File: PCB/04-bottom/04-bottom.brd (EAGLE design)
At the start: 128 x 129.5 mm, 30 parts, among them CN1 ML8-R, J1 5267-3, J2 5267-3, J3 5267-3, J4 5267-3, J5 22057045, J6 22057045, J7 5267-3

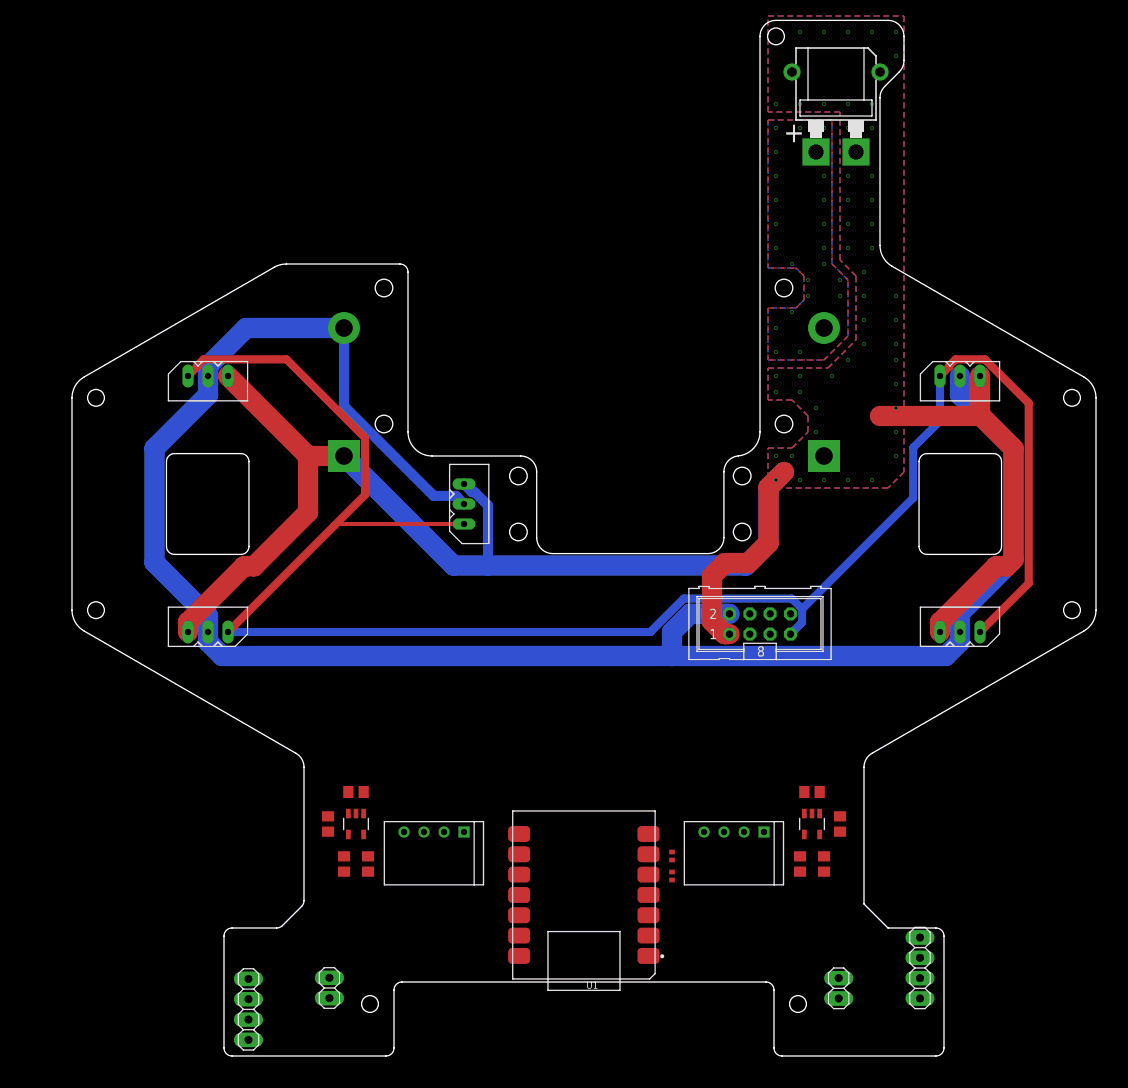
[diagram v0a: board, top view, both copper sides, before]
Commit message: 配線完了！！
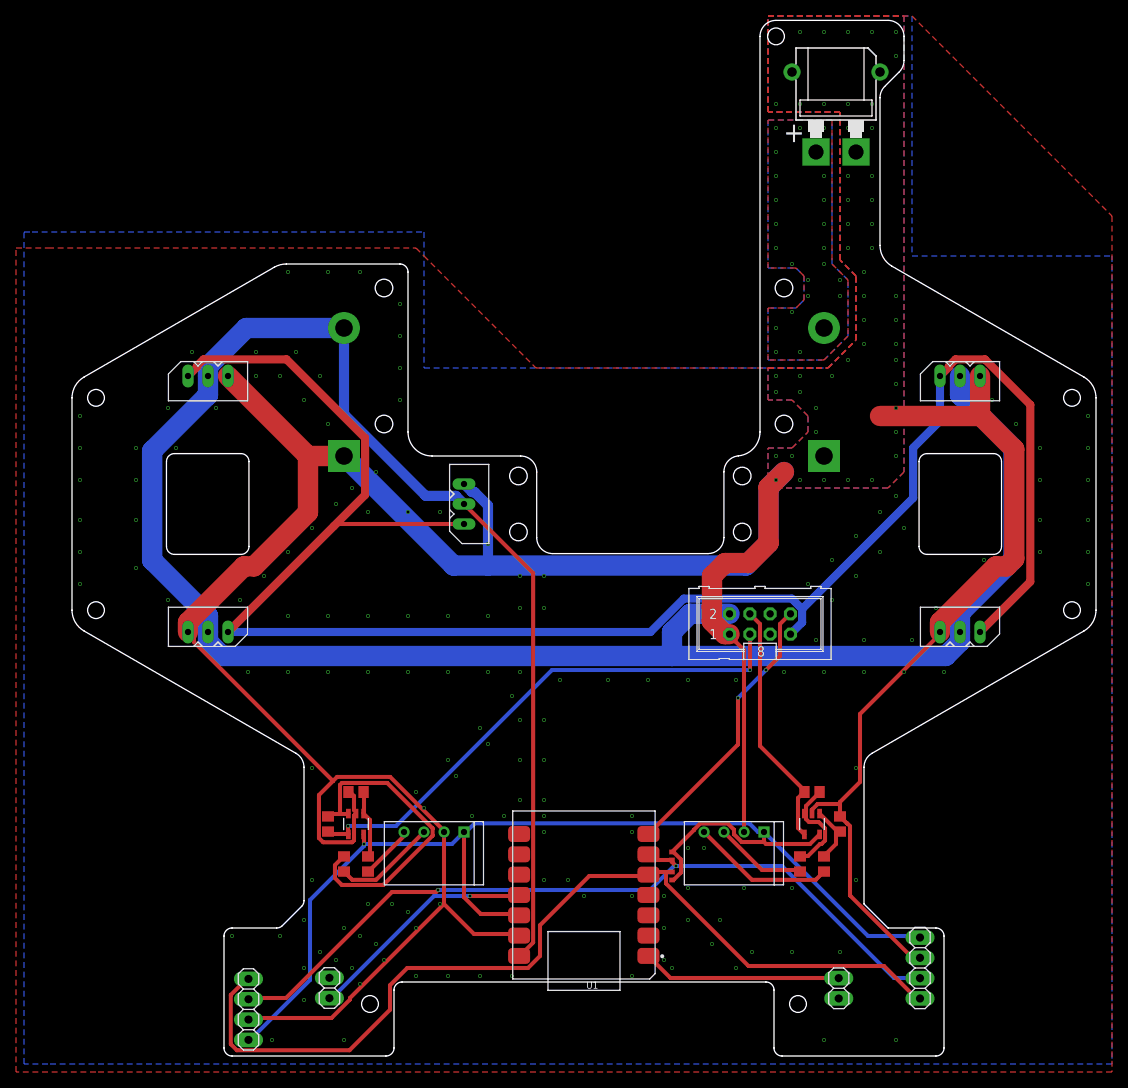
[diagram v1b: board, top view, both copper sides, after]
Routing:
- net GND: track 206.7 -> 400.1 mm, vias 48 -> 212
- net +3V3: track 0.00 -> 152.0 mm, vias 0 -> 1
- net SDA: track 0.00 -> 117.2 mm
- net SCL: track 0.00 -> 101.1 mm, vias 0 -> 2
- net LOADCELL-R: track 0.00 -> 66.7 mm, vias 0 -> 2
- net VDD: track 234.2 -> 295.8 mm
- net N$7: track 0.00 -> 39.8 mm
- net MIRROR: track 0.00 -> 34.9 mm, vias 0 -> 2
- net LOADCELL-L: track 0.00 -> 31.1 mm
- net XSHUT1: track 0.00 -> 29.1 mm, vias 0 -> 1
- net XSHUT2: track 0.00 -> 24.9 mm
- net N$2: track 0.00 -> 17.9 mm
- net N$5: track 0.00 -> 12.9 mm
- net N$3: track 0.00 -> 12.6 mm
- net N$1: track 0.00 -> 11.6 mm
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
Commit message: Revert "配線完了！！"
This reverts commit 358a7b28429e96d6d805ade8accdc2bc4b7907af.
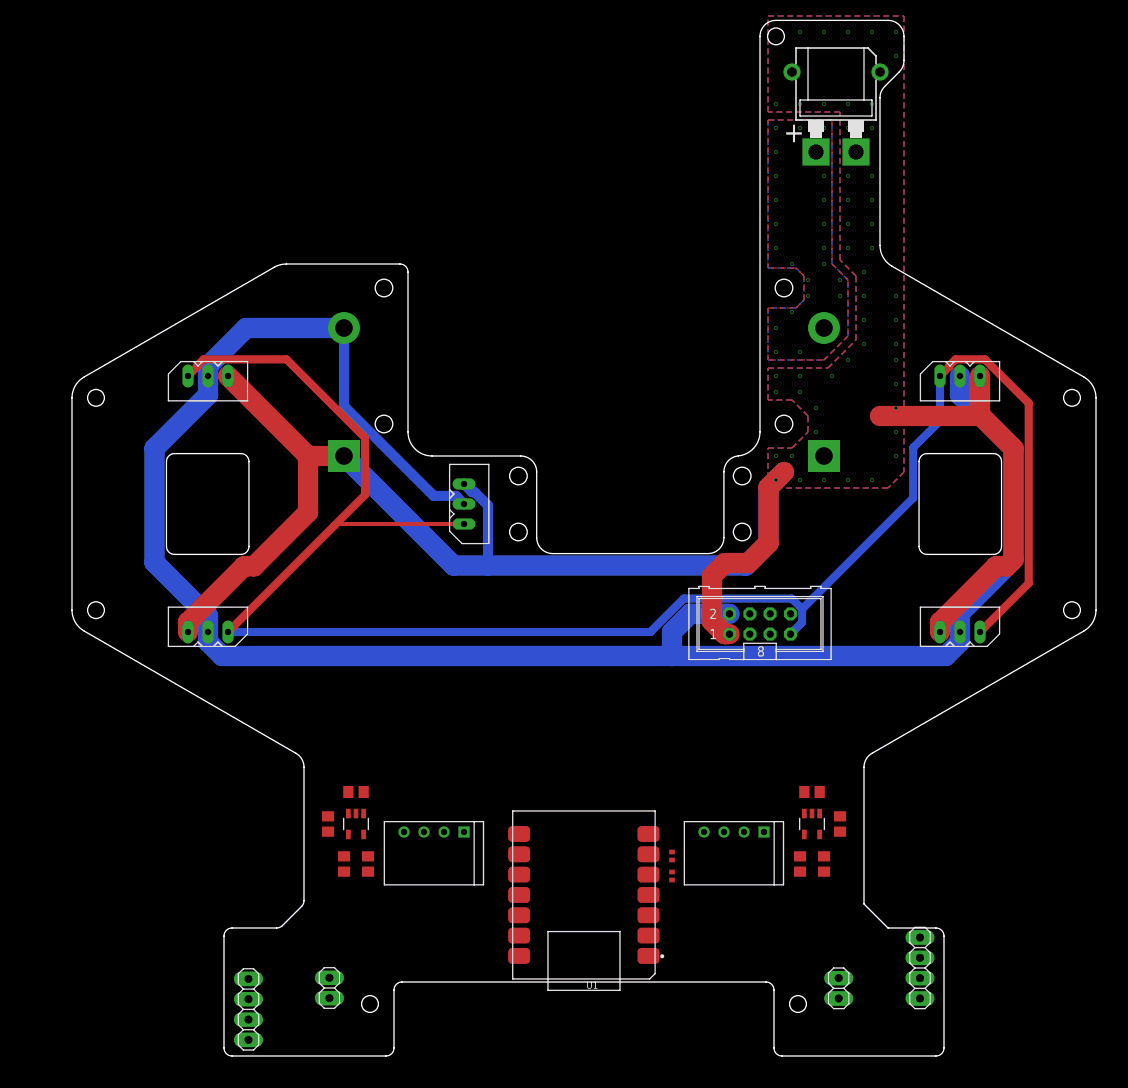
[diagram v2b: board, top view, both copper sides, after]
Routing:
- net GND: track 400.1 -> 206.7 mm, vias 212 -> 48
- net +3V3: track 152.0 -> 0.00 mm, vias 1 -> 0
- net SDA: track 117.2 -> 0.00 mm
- net SCL: track 101.1 -> 0.00 mm, vias 2 -> 0
- net LOADCELL-R: track 66.7 -> 0.00 mm, vias 2 -> 0
- net VDD: track 295.8 -> 234.2 mm
- net N$7: track 39.8 -> 0.00 mm
- net MIRROR: track 34.9 -> 0.00 mm, vias 2 -> 0
- net LOADCELL-L: track 31.1 -> 0.00 mm
- net XSHUT1: track 29.1 -> 0.00 mm, vias 1 -> 0
- net XSHUT2: track 24.9 -> 0.00 mm
- net N$2: track 17.9 -> 0.00 mm
- net N$5: track 12.9 -> 0.00 mm
- net N$3: track 12.6 -> 0.00 mm
- net N$1: track 11.6 -> 0.00 mm
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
